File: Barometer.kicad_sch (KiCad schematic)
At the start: 2 parts, among them U1 BMP280

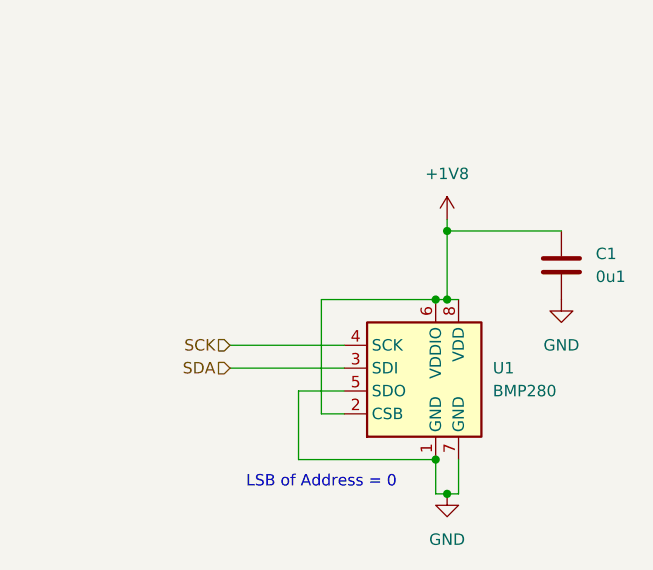
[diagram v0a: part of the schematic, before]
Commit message: deleted demo
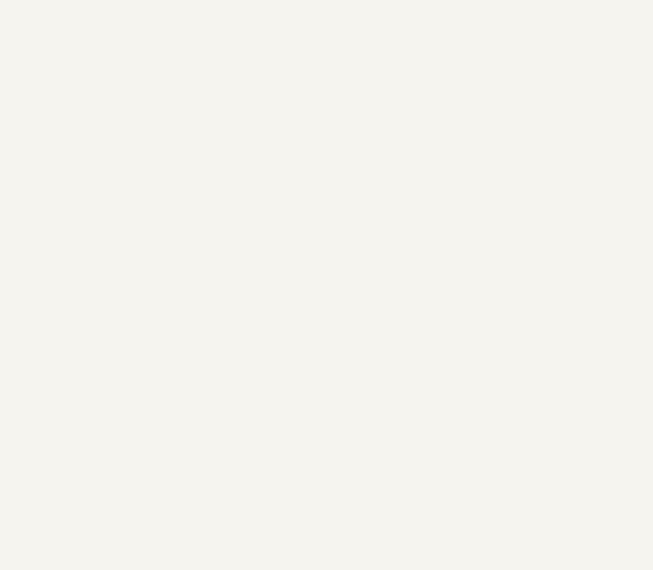
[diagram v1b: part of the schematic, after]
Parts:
- removed C1: 0u1, Capacitor_SMD:C_0603_1608Metric, symbol Device:C
- removed U1: BMP280, Package_LGA:Bosch_LGA-8_2x2.5mm_P0.65mm_ClockwisePinNumbering, symbol Sensor_Pressure:BMP280
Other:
- note removed: "LSB of Address = 0"

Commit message: barometer test
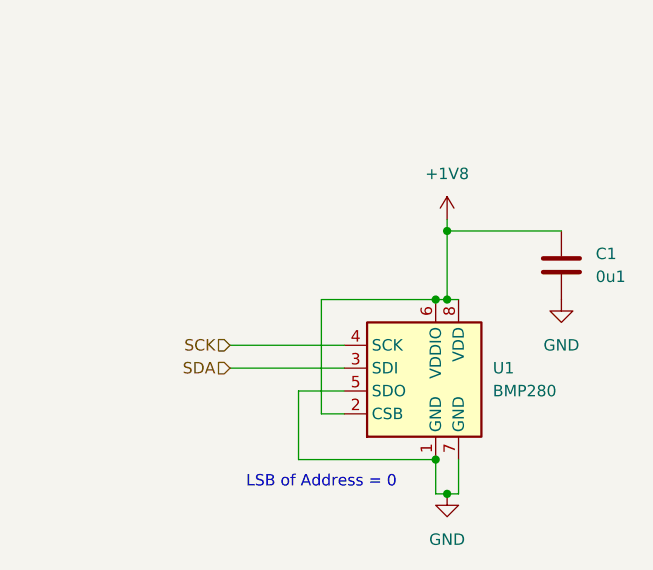
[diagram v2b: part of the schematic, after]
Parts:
- added C1: 0u1, Capacitor_SMD:C_0603_1608Metric, symbol Device:C
- added U1: BMP280, Package_LGA:Bosch_LGA-8_2x2.5mm_P0.65mm_ClockwisePinNumbering, symbol Sensor_Pressure:BMP280
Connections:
- new net +1V8: C1.1, U1.2 (CSB), U1.6 (VDDIO), U1.8 (VDD)
- new net GND: C1.2, U1.1 (GND), U1.5 (SDO), U1.7 (GND)
- new net SCK: U1.4 (SCK)
- new net SDA: U1.3 (SDI)
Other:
- note added: "LSB of Address = 0"
